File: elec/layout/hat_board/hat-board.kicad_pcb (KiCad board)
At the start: 4 copper layers, 108 x 115.9 mm, 82 parts, among them P1 HatButtonAntenna, U1 _NXP_Semicon_PN5321A3HN_C106_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, U10 _OPSCO_Optoelectronics_SK6805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, U11 _OPSCO_Optoelectronics_SK6805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, U12 _OPSCO_Optoelectronics_SK6805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, U13 _OPSCO_Optoelectronics_SK6805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, U14 _OPSCO_Optoelectronics_SK6805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, U15 _OPSCO_Optoelectronics_SK6805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, U16 _OPSCO_Optoelectronics_SK6805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, U17 _OPSCO_Optoelectronics_SK6805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, U18 _OPSCO_Optoelectronics_SK6805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, U19 _OPSCO_Optoelectronics_SK6805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, U2 _OPSCO_Optoelectronics_SK6805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, U20 _OPSCO_Optoelectronics_SK6805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, U21 _OPSCO_Optoelectronics_SK6805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, U22 _OPSCO_Optoelectronics_SK6805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, U23 _OPSCO_Optoelectronics_SK6805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, U24 _OPSCO_Optoelectronics_SK6805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, U25 _Microchip_Tech_CAP1188_1_CP_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, U3 _OPSCO_Optoelectronics_SK6805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, U4 _OPSCO_Optoelectronics_SK6805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, U5 _OPSCO_Optoelectronics_SK6805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, U6 _OPSCO_Optoelectronics_SK6805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, U7 _OPSCO_Optoelectronics_SK6805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, U8 _OPSCO_Optoelectronics_SK6805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, U9 _OPSCO_Optoelectronics_SK6805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

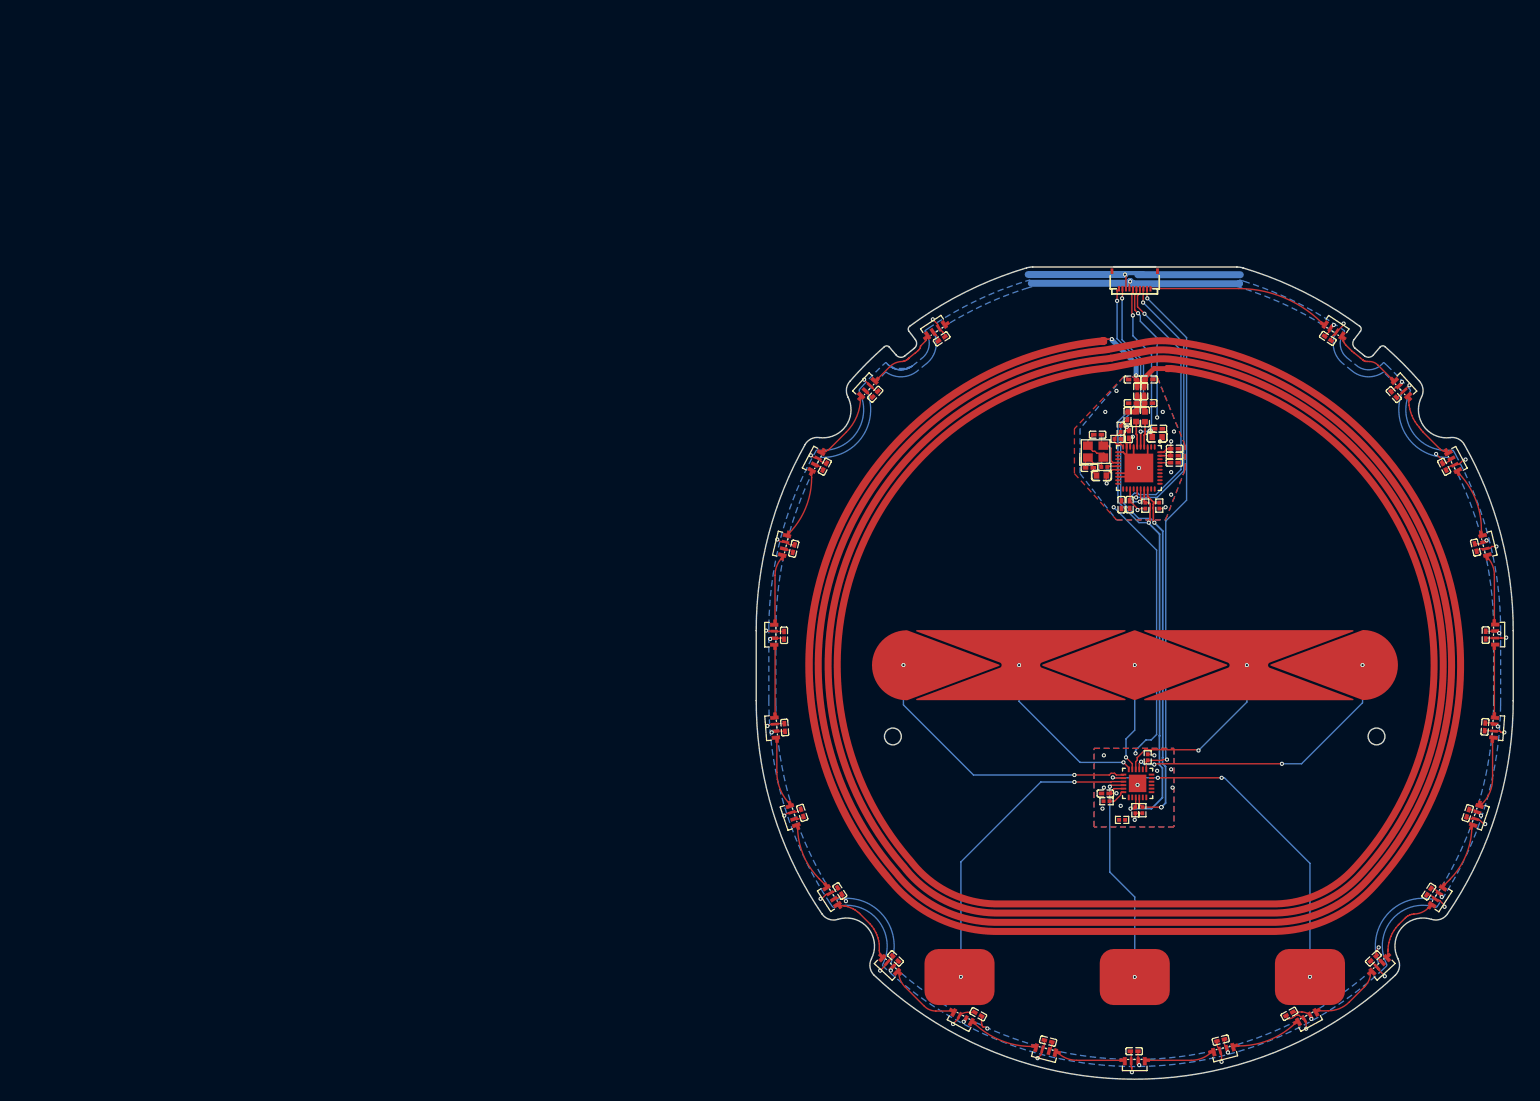
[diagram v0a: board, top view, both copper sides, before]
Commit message: Build full
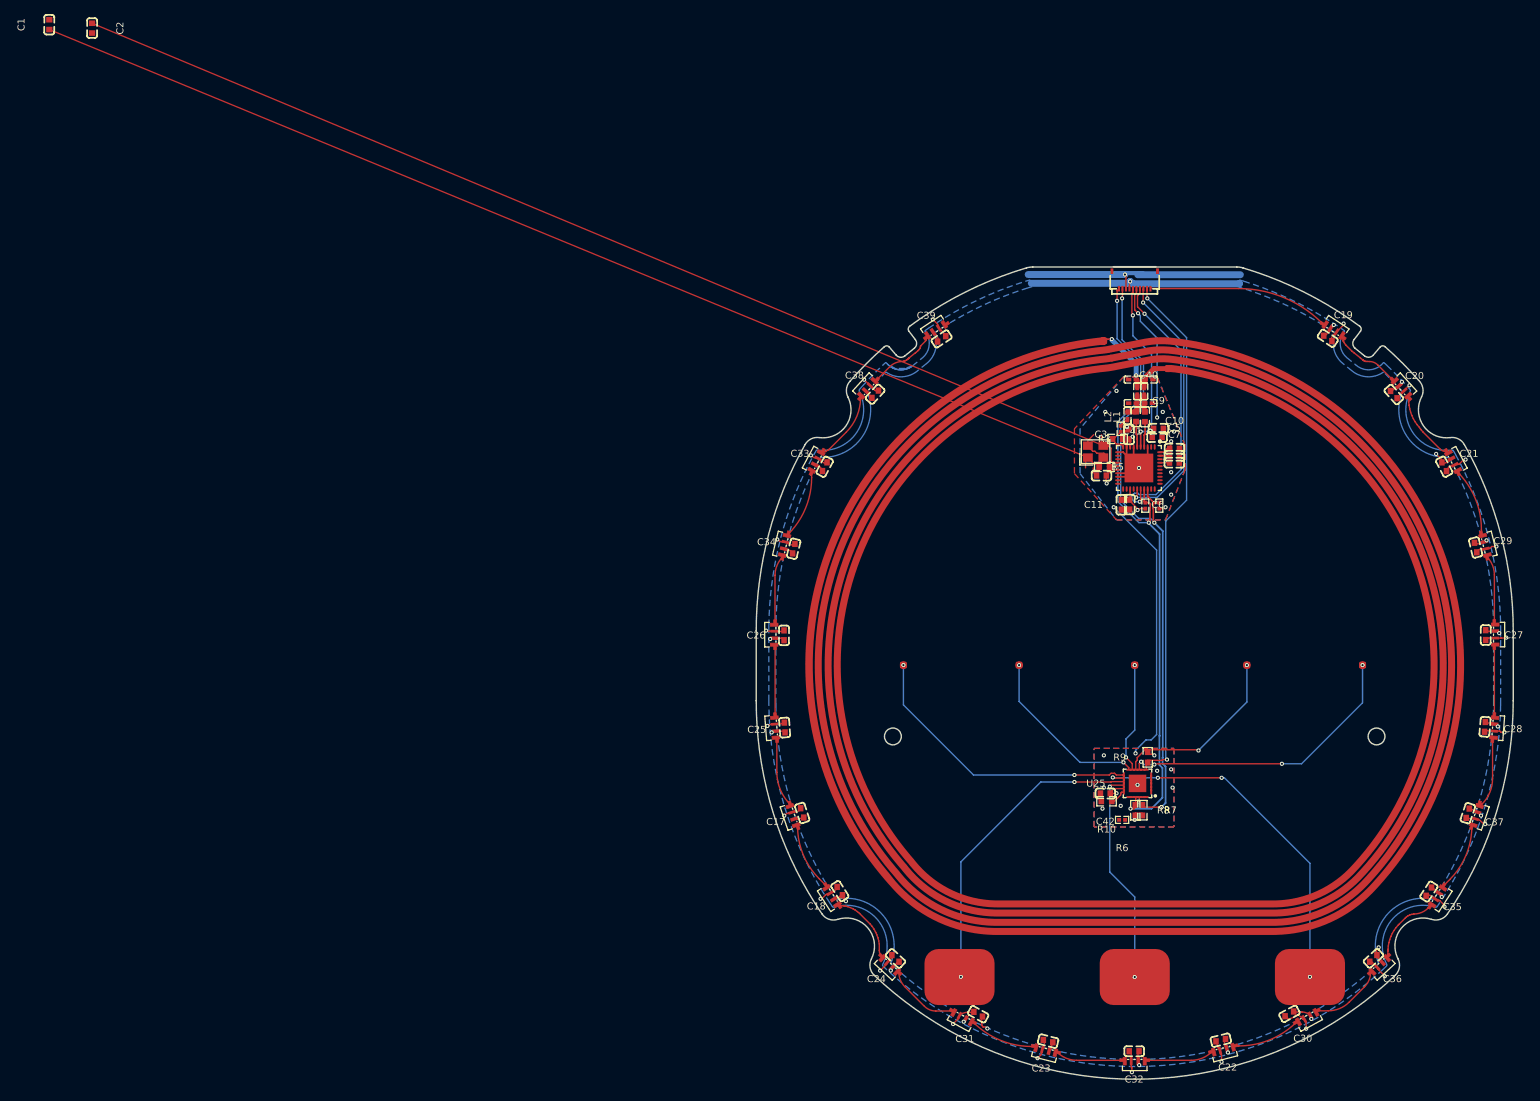
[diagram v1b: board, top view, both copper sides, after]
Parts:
- C1, C2: value 20pF ±5% 50V C0G -> 100nF ±10% 50V X7R; footprint lcsc:C0402 -> lcsc:C0603
- C10, C11, C17, C18, C19, C20, C21, C22, C23, C24, C25, C26, C27, C28, C29, C3, C30, C31, C32, C33, C34, C35, C36, C37, C38, C39, C42, C5, C6, C7, C9: value 100nF ±10% 16V X7R -> 100nF ±10% 50V X7R; footprint lcsc:C0402 -> lcsc:C0603
- C4, C8: value 10µF ±10% 10V X5R -> 100nF ±10% 50V X7R
- L1, L2: value 560nH ±5% 450mA 480mΩ -> 560nH ±5% infHz 450mA 480mΩ
- R1, R2: value 5.1kΩ ±1% 62.5mW -> 10kΩ ±1% 62.5mW
- R10, R9: value 10kΩ ±1% 62.5mW -> 1kΩ ±1% 100mW; footprint lcsc:R0402 -> lcsc:R0603
- R3, R5, R7, R8: value 5.1kΩ ±1% 62.5mW -> 1kΩ ±1% 100mW; footprint lcsc:R0402 -> lcsc:R0603
- U25: footprint lcsc:QFN-24_L4.0-W4.0-P0.50-TL-EP2.5 -> lcsc:QFN-24_L4.0-W4.0-P0.50-BL-EP2.5
- moved C1 161.3 mm to (-3.05, -0.25), turned to 90 degrees
- moved C2 154.7 mm to (3.05, 0.25), turned to 270 degrees
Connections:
- C10 pad 1: power_3v3 -> power_5v
- C11 pad 1: gnd -> power_5v
- C11 pad 2: lv -> gnd
- C12 pad 2: nfc-net -> nfc-net-6
- C2 pad 1: nfc-net-3 -> nfc-net
- C32 pad 1: power_5v -> power_3v3
- C33 pad 1: power_5v -> power_3v3
- C34 pad 1: power_5v -> power_3v3
- C35 pad 1: power_5v -> power_3v3
- C36 pad 1: power_5v -> nfc-net-2
- C37 pad 1: power_5v -> power_3v3
- C38 pad 1: power_5v -> power_3v3
- C39 pad 1: power_5v -> power_3v3
- C4 pad 1: power_3v3 -> power_5v
- C42 pad 1: power_3v3 -> gnd
- C42 pad 2: gnd -> lv
- C5 pad 1: power_3v3 -> power_5v
- C6 pad 1: power_3v3 -> power_5v
- C7 pad 1: nfc-net-4 -> power_5v
- C8 pad 1: power_3v3 -> power_5v
- C9 pad 1: power_3v3 -> power_5v
- L1 pad 2: nfc-net-2 -> nfc-net-1
- R1 pad 1: i2c_scl -> capacitive_sensor-net-1
- R1 pad 2: power_3v3 -> gnd
- R10 pad 1: capacitive_sensor-net -> i2c_sda
- R10 pad 2: gnd -> power_3v3
- R2 pad 1: i2c_sda -> capacitive_sensor-net
- R2 pad 2: power_3v3 -> gnd
- R3 pad 2: nfc-net-6 -> nfc-net-3
- R4 pad 1: nfc-net -> nfc-net-6
- R4 pad 2: nfc-net-1 -> nfc-net-4
- R5 pad 2: nfc-net-1 -> nfc-net-4
- R6 pad 1: capacitive_sensor.address-signal -> touch_irq
- R6 pad 2: gnd -> power_3v3
- R9 pad 1: touch_irq -> i2c_scl
- U1 pad 10: nfc-net-1 -> nfc-net-4
- U1 pad 14: nfc-net-3 -> nfc-net
- U1 pad 15: nfc-net-6 -> nfc-net-3
- U1 pad 20: nfc.nfc_ic-net -> nfc.nfc_ic.footprint.pins[12].net-net
- U1 pad 21: nfc.nfc_ic-net -> nfc.nfc_ic.footprint.pins[13].net-net
- U1 pad 22: nfc.nfc_ic-net -> nfc.nfc_ic.footprint.pins[14].net-net
- U1 pad 37: nfc-net-4 -> nfc-net-2
- U1 pad 4: nfc-net-2 -> nfc-net-1
- U10 pad 1: signal-1 -> signal-17
- U10 pad 4: signal-16 -> signal-19
- U11 pad 1: signal -> signal-16
- U11 pad 4: signal-1 -> signal-17
- U12 pad 1: signal-9 -> signal-21
- U12 pad 4: signal -> signal-16
- U13 pad 1: signal-6 -> signal-9
- U13 pad 4: signal-7 -> signal-10
- U14 pad 1: signal-8 -> signal-11
- U14 pad 4: signal-9 -> signal-21
- U15 pad 1: signal-21 -> signal
- U15 pad 4: signal-8 -> signal-11
- U16 pad 4: signal-21 -> signal
- U17 pad 1: signal-12 -> signal-20
- U17 pad 4: signal-6 -> signal-9
- U18 pad 1: signal-18 -> signal-15
- U18 pad 4: signal-12 -> signal-20
- U19 pad 1: signal-5 -> signal-2
- U19 pad 4: signal-18 -> signal-15
- U2 pad 1: signal-7 -> signal-10
- U20 pad 1: signal-4 -> signal-1
- U20 pad 4: signal-5 -> signal-2
- U21 pad 1: signal-11 -> signal-6
- U21 pad 4: signal-4 -> signal-1
- U22 pad 1: signal-10 -> signal-5
- U22 pad 4: signal-11 -> signal-6
- U23 pad 1: signal-13 -> signal-4
- U23 pad 4: signal-10 -> signal-5
- U24 pad 1: signal-15 -> signal-3
- U24 pad 4: signal-13 -> signal-4
- U25 pad 14: addr_comm -> capacitive_sensor-net-1
- U3 pad 1: signal-20 -> signal-18
- U3 pad 4: signal-15 -> signal-3
- U4 pad 4: signal-20 -> signal-18
- U5 pad 1: signal-3 -> signal-13
- U6 pad 1: signal-2 -> signal-8
- U6 pad 4: signal-3 -> signal-13
- U7 pad 1: signal-19 -> signal-7
- U7 pad 4: signal-2 -> signal-8
- U8 pad 1: signal-17 -> signal-12
- U8 pad 4: signal-19 -> signal-7
- U9 pad 1: signal-16 -> signal-19
- U9 pad 4: signal-17 -> signal-12
- XTAL1 pad 3: nfc-net-3 -> nfc-net
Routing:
- net nfc.oscillator-net: track 6.65 -> 166.9 mm
- net nfc-net: track 1.57 -> 157.9 mm
